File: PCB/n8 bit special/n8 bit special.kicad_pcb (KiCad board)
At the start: 4 copper layers, 99.9 x 100 mm, 50 parts, among them J1 USB_B_Micro, J2 PORT0, J3 PORT1, J4 PORT2, J6 Conn_02x08_Odd_Even, Q1 2N3904, SW1 SW_Push_Dual, U1 W65C02SxP, U10 74HC00, U2 CY62256-70PC, U3 CY62256-70PC, U4 28C256, U5 SC28L92_PLC44, U6 22V10C, U7 DS1813, U8 CH340C, U9 74LS21, X1 3.6864Mhz

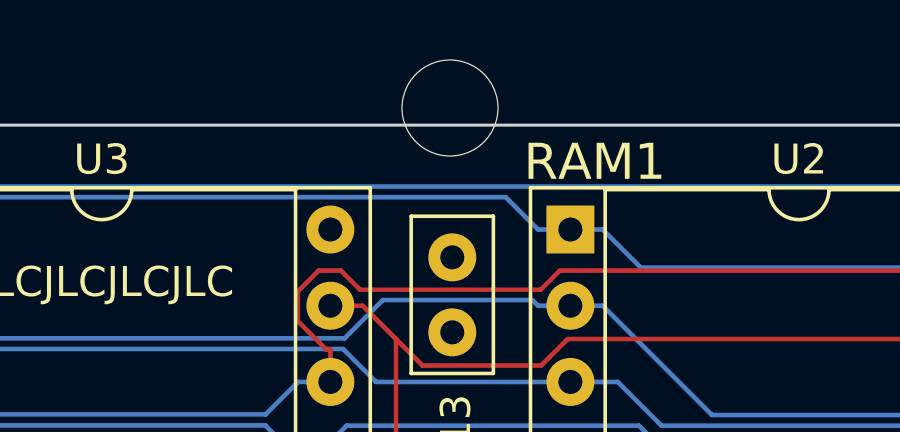
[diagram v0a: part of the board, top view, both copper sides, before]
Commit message: rc1 before library swap test
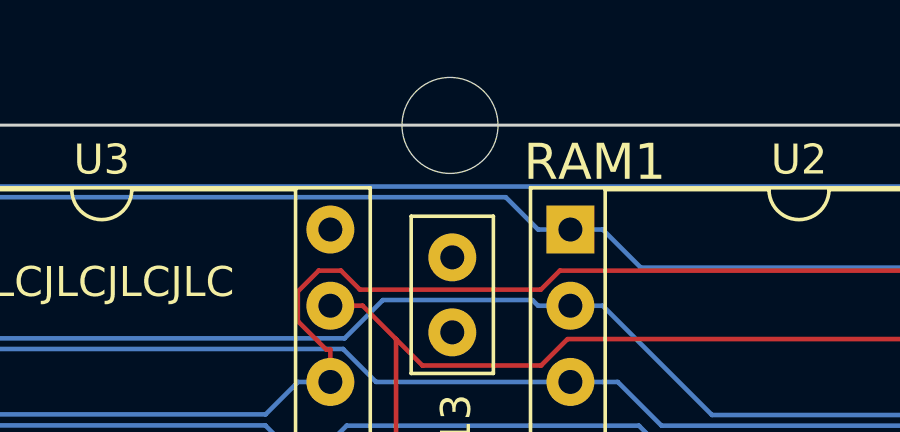
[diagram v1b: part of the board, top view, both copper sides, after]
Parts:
- moved REF** 0.58 mm to (133.1, 39.9)
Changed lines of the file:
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@@
   )
   (footprint "MountingHole:MountingHole_3.2mm_M3" (layer "F.Cu")
-    (at 133.1468 39.3192)
+    (at 133.1468 39.9)
     (descr "Mounting Hole 3.2mm, no annular, M3")
     (tags "mounting hole 3.2mm no annular m3")
